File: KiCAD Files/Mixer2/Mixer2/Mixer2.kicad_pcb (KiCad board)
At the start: 4 copper layers, 59 x 30.5 mm, 83 parts, among them IC1 FST3253MTCX, K1 G6K-2F-Y DC3, U1 BGA420H6327XTSA1, U2 Si5351A-B-GT, U3 SN74AC74PWR, U4 TXU0101DBVR, U5 4053, U6 4053, U7 OPA1678IDGKT, U8 OPA1678IDGKT, U9 OPA1678IDGKT, Y1 ECS-250-8-30B-CKM

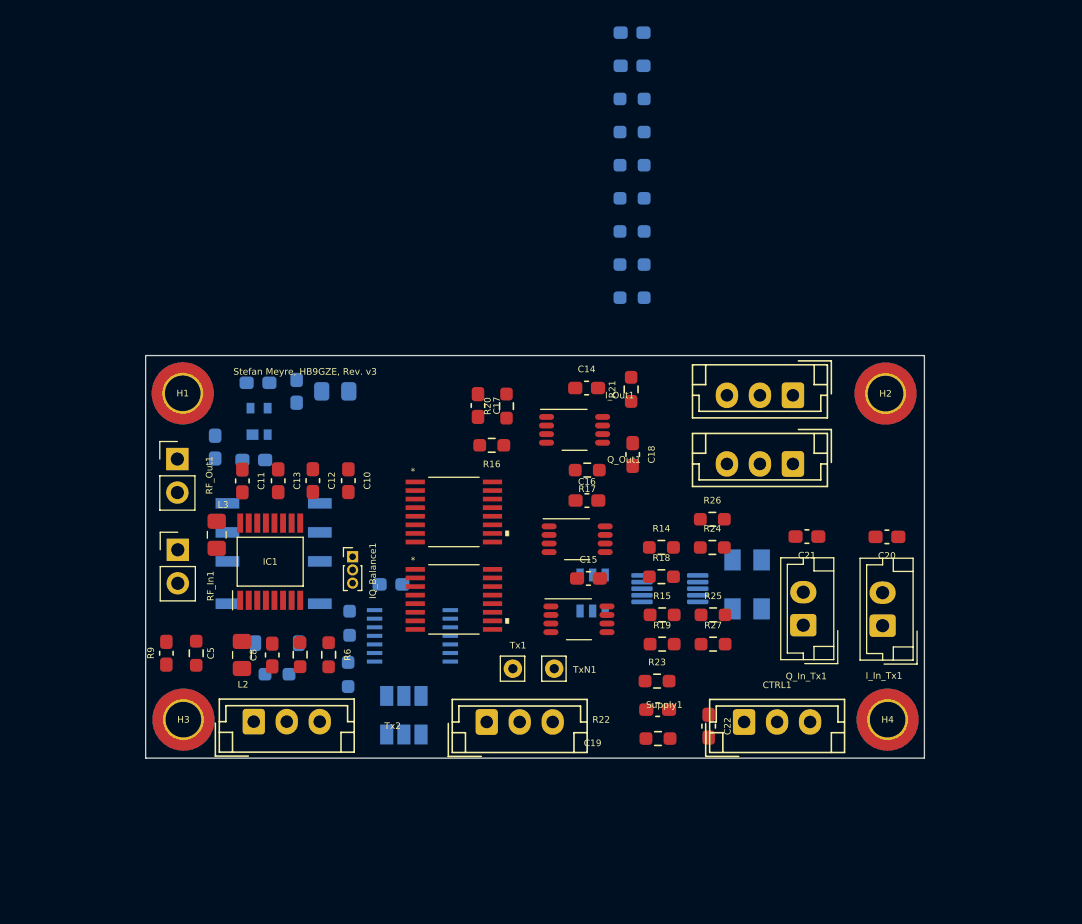
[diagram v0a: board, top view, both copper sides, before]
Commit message: final mixer2 board
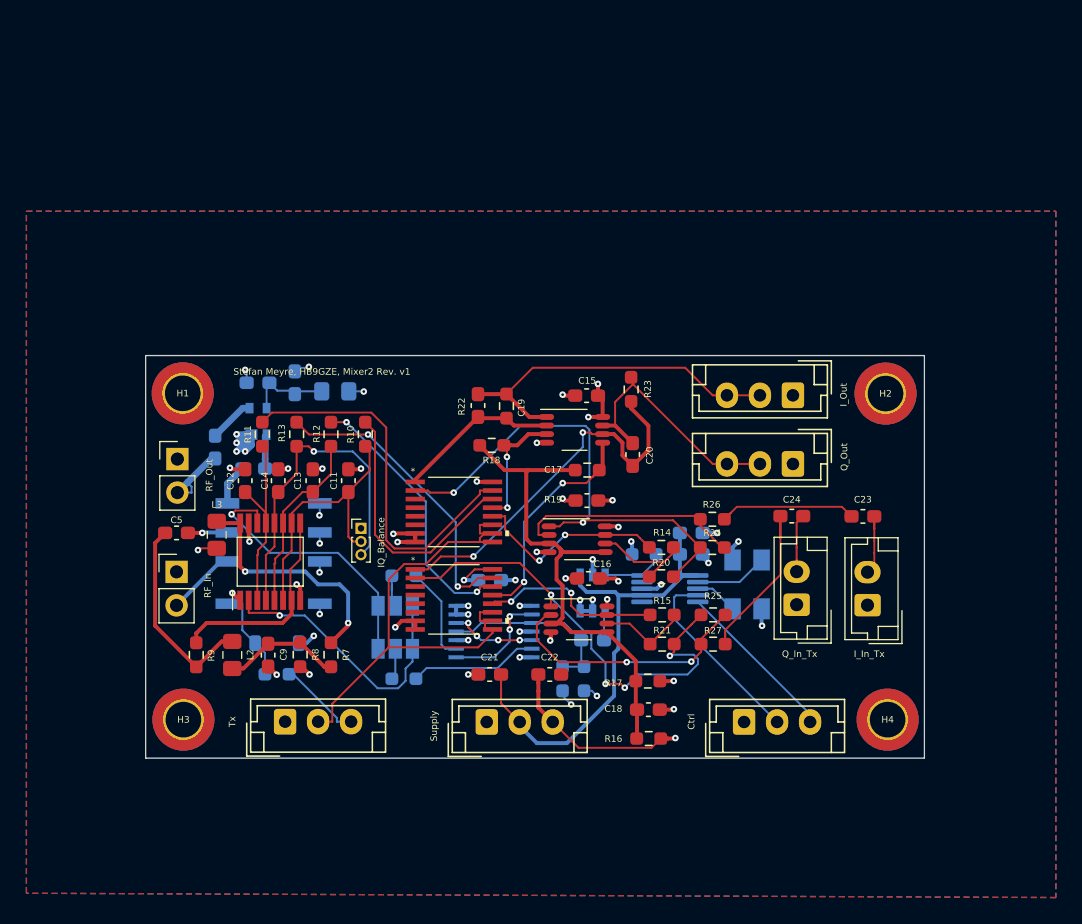
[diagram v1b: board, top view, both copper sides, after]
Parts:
- removed Tx1, TxN1: TestPoint, Connector_Pin:Pin_D0.7mm_L6.5mm_W1.8mm_FlatFork
- added C10: 100nF, Capacitor_SMD:C_0603_1608Metric_Pad1.08x0.95mm_HandSolder, B.Cu at (133.9, 71.5)
- added C21: 100nF, Capacitor_SMD:C_0603_1608Metric_Pad1.08x0.95mm_HandSolder, F.Cu at (126.1, 74.1)
- R10, R11, R12, R13: moved to F.Cu
- R16: renamed from R22; value 1k -> 10k
- R17: renamed from R23; value 1k -> 10k
- R5: renamed from R4; value 47R -> DNF
- moved R3 44.1 mm to (133.2, 74.4), turned to -90 degrees
- moved C2 39.8 mm to (141.4, 65.0)
- moved R4 39.3 mm to (131.6, 74.4), turned to 90 degrees
- moved C3 35.7 mm to (141.4, 63.4)
- moved R5 32.0 mm to (137.8, 65.0)
- moved R11 31.9 mm to (108.9, 55.9), turned to 90 degrees
- moved R13 27.4 mm to (111.5, 55.9), turned to 90 degrees
- moved R10 27.0 mm to (116.7, 55.9), turned to 90 degrees
- moved R12 26.2 mm to (114.1, 55.9), turned to 90 degrees
- moved C22 12.7 mm to (130.7, 74.1), turned to 180 degrees
- moved JP2 9.77 mm to (119.0, 68.9)
- moved C5 9.15 mm to (102.4, 63.4), turned to 180 degrees
- moved C6 7.48 mm to (126.1, 67.0)
- moved U2 6.18 mm to (126.4, 70.8)
- moved R6 5.46 mm to (119.6, 66.6), turned to 0 degrees
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- renumbered C3 to C1, C10 to C11, C11 to C12, C12 to C13, C13 to C14, C14 to C15, C15 to C16, C16 to C17, C19 to C18, C17 to C19, C1 to C2, C18 to C20, C20 to C23, C21 to C24, C2 to C3, C9 to C6, C6 to C7, C7 to C8, C8 to C9, CTRL1 to Ctrl, IQ_Balance1 to IQ_Balance, I_In_Tx1 to I_In_Tx, I_Out1 to I_Out, Q_In_Tx1 to Q_In_Tx, Q_Out1 to Q_Out, R16 to R18, R17 to R19, R18 to R20, R19 to R21, R20 to R22, R21 to R23, R5 to R4, R8 to R6, R6 to R7, R7 to R8, RF_In1 to RF_In, RF_Out1 to RF_Out, Supply1 to Supply, Tx2 to Tx, U3 to U2, U2 to U3
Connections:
- U4 pad 4: /SI5351CLK -> Net-(U4-BY)
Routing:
- net GND: track 0.00 -> 50.0 mm, vias 0 -> 42
- net +5V: track 0.00 -> 44.0 mm, vias 0 -> 19
- net /+2.5V: track 0.00 -> 39.4 mm
- net Net-(U5-Y0): track 0.00 -> 39.3 mm, vias 0 -> 2
- net +3.3V: track 0.00 -> 39.2 mm
- net /Tx: track 0.00 -> 38.6 mm
- net Net-(U6-Y0): track 0.00 -> 36.6 mm, vias 0 -> 4
- net Net-(U6-Y1): track 0.00 -> 29.3 mm, vias 0 -> 2
- net Net-(U5-Y): track 0.00 -> 29.0 mm
- net Net-(I_Out1-Pin_2): track 0.00 -> 26.8 mm
- net /3: track 0.00 -> 25.7 mm, vias 0 -> 1
- net Net-(U6-Y): track 0.00 -> 23.0 mm, vias 0 -> 2
- net Net-(U9A-IN-): track 0.00 -> 21.6 mm, vias 0 -> 2
- net /S1: track 0.00 -> 21.3 mm, vias 0 -> 1
- net /S0: track 0.00 -> 20.8 mm, vias 0 -> 1
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- added copper zone on In2.Cu, net +5V
- added copper zone on B.Cu, net GND
- added copper zone on F.Cu, net GND
- added copper zone on In1.Cu, net GND
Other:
- board text added: "Stefan Meyre, HB9GZE, Mixer2 Rev. v1"
- board text removed: "${REFERENCE}"
- board text removed: "Stefan Meyre, HB9GZE, Rev. v3"
